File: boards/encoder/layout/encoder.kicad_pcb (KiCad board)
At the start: 2 copper layers, 9.6 x 14.1 mm, 3 parts, among them IC1 AS5047U-HTSM, J1 EncoderTab

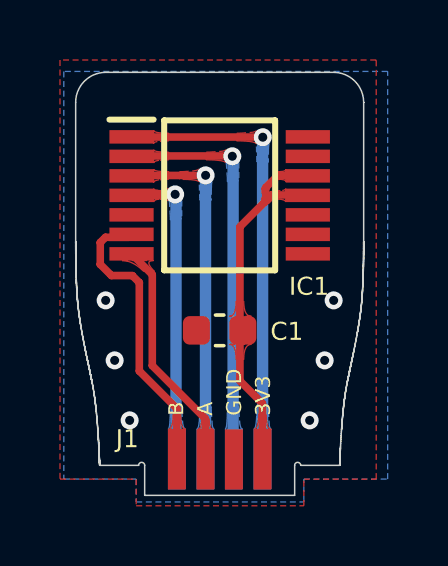
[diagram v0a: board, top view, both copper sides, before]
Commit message: 🚚 Transfer the Altium pour, teardrop and outline settings to the layouts
The transfer scripts now carry what KiCad's Altium importer drops, and
the layouts are regenerated with them:

- Teardrops (converted to plain zones) fill with a 0.1 mm minimum width
  instead of the importer's 0.25 mm, which left 652 of 786 (main), 5 of
  25 (encoder) and 10 of 46 (bluetooth) teardrops without copper. 0.1 mm
  is JLCPCB's minimum copper feature: 0.0254 mm fills slightly more but
  fails the DFM feature width on all three boards.
- Pours use the Altium polygons' neck width as minimum width (0.1 mm;
  0.4 mm on the encoder's bottom pour, which keeps it out of the channels
  between the SPI tracks, 0.3 mm on the bluetooth plug pour).
- Inner-layer pours relieve through-hole pads (0.254 mm spokes and gap,
  Altium rule PolygonConnect); outer pours stay solid.
- Main In1/In2 keep Altium's 1.559 / 2.074 mm voids around H1-H4
  (copper-pour keepouts).
- Edge.Cuts lines under 1 um (main 6, encoder 1, bluetooth 7) are left
  out and their neighbours joined, so KiCad reads the outlines as valid.
- The board mask expansion is copied from the previous board (0.02 mm);
  main takes the spec's aux origin.
- D4/D5 and bluetooth D1 3D models are scaled to the datasheet heights.
- rework.py catches all six teardrops of the removed C1 VBAT chain (three
  were left as stubs, invisible while unfilled).
- The encoder drops an embedded TSSOP-14 STEP no footprint uses; the
  bluetooth script calls previous.altium_pcb (renamed).

The main layout footprints were resynced from their packages
(pcb layout --sync-footprints), which brings the new WallSensor
silkscreen, R31-R33 and U2's keepouts on all four copper layers.
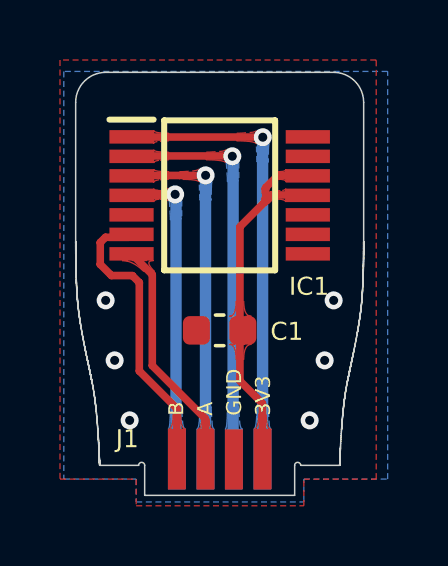
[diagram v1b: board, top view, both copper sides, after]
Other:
- rule pad_to_mask_clearance: 0 -> 0.02
